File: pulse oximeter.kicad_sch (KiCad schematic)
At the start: 24 parts, among them J1 USB_C_Receptacle_USB2.0_14P, J2 Conn_01x04_Socket, J3 Conn_01x02_Socket, Q1 FS8205A, SW1 SW_Push, SW2 RESET, U1 ATMEGA328P-AU, U2 AP2112K-3.3TRG1, U3 DW01A, U4 MAX30102EFD_, U5 MCP73831-2-OT, U6 CH340C, Y1 8MHz

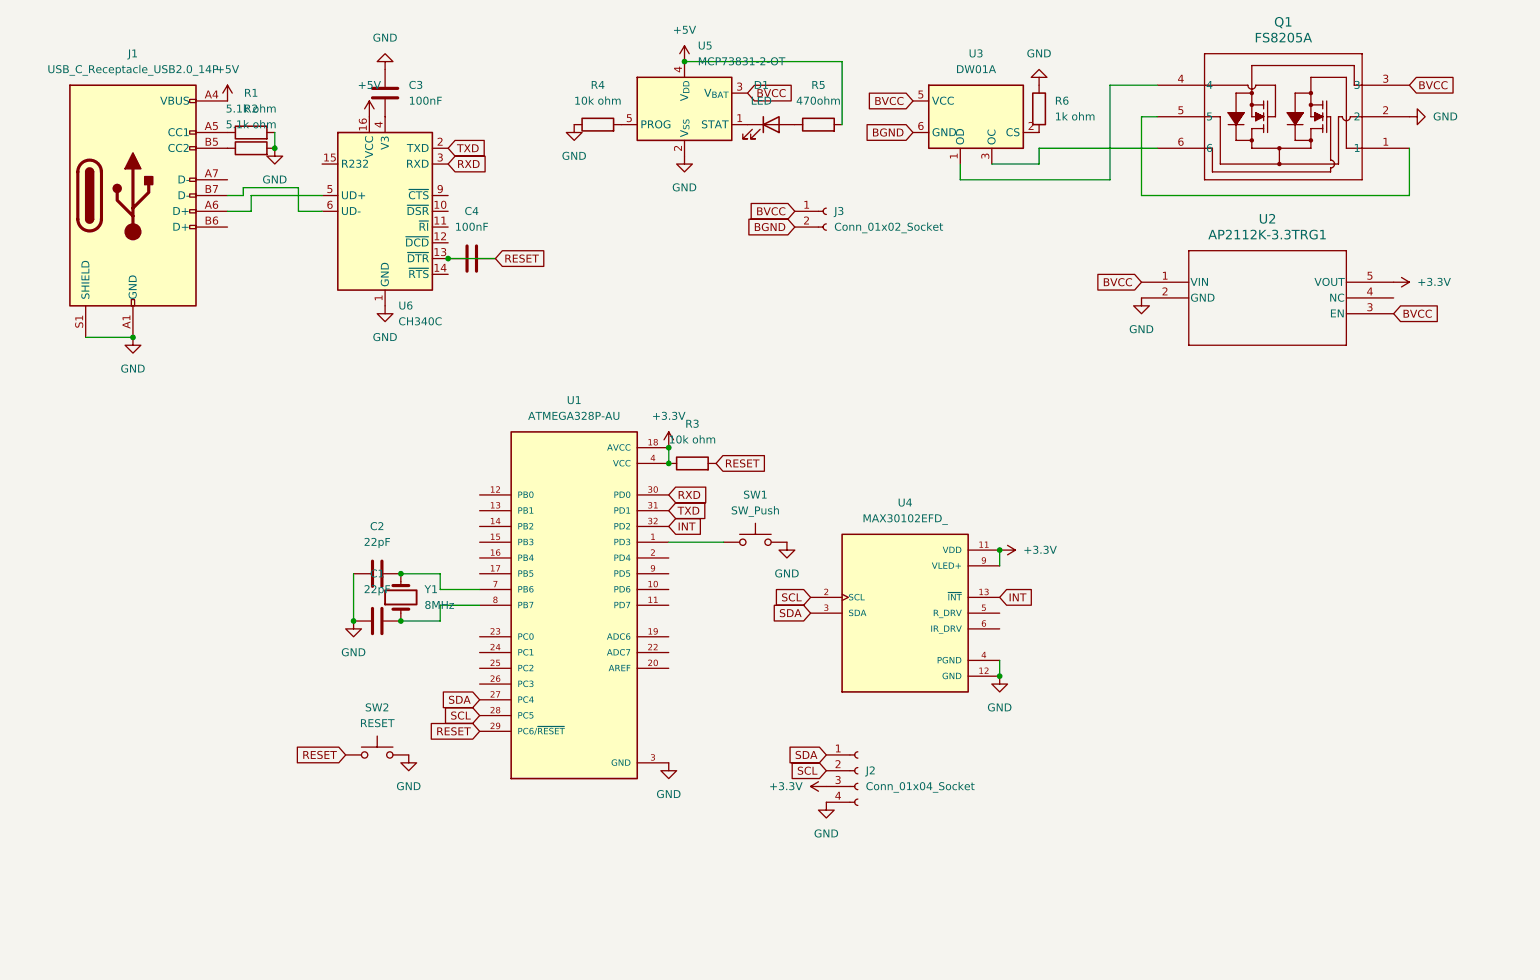
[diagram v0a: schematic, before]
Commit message: Edit PCB and Schematic
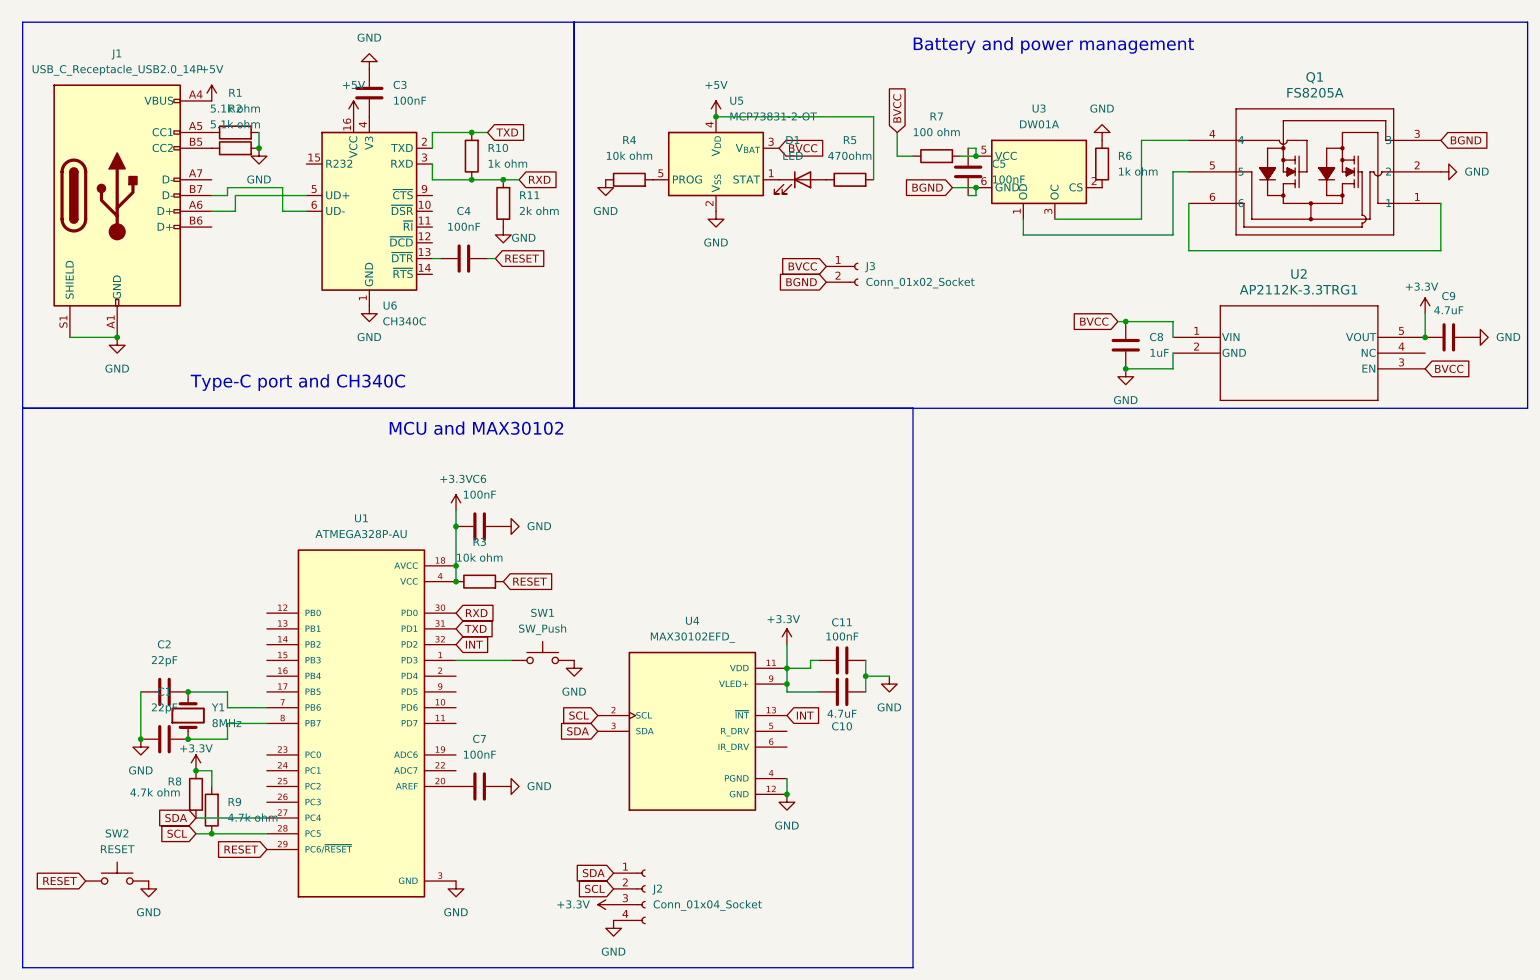
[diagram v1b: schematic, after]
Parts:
- added C10, C9: 4.7uF, Capacitor_SMD:C_0603_1608Metric, symbol Device:C
- added C11, C5, C6, C7: 100nF, Capacitor_SMD:C_0603_1608Metric, symbol Device:C
- added C8: 1uF, Capacitor_SMD:C_0603_1608Metric, symbol Device:C
- added R10: 1k ohm, Resistor_SMD:R_0603_1608Metric, symbol Device:R
- added R11: 2k ohm, Resistor_SMD:R_0603_1608Metric, symbol Device:R
- added R7: 100 ohm, Resistor_SMD:R_0603_1608Metric, symbol Device:R
- added R8, R9: 4.7k ohm, Resistor_SMD:R_0603_1608Metric, symbol Device:R
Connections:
- net +3.3V: now also C10.1, C11.1, C6.1, C9.1, R8.1, R9.2
- net BGND: now also Q1.3, C5.2
- net BVCC: now also C8.1, R7.1; no longer Q1.3, U3.5 (VCC)
- net GND: now also C10.2, C11.2, C6.2, C7.2, C8.2, C9.2, R11.1
- net RESET: no longer C4.2, U6.13 (~{DTR})
- net RXD: now also R10.1, R11.2
- net SCL: now also R9.1
- net SDA: now also R8.2
- net TXD: now also R10.2
- net at Q1.1: now also Q1.6; no longer Q1.5
- net at Q1.4: now also U3.3 (OC); no longer U3.1 (OD)
- net at U1.20 (AREF): now also C7.1
- new net: Q1.5, U3.1 (OD)
- new net: C5.1, R7.2, U3.5 (VCC)
- new net: C4.2, U6.13 (~{DTR})
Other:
- note added: "Battery and power management"
- note added: "MCU and MAX30102"
- note added: "Type-C port and CH340C"
- moved on the sheet: C1, C2, C3, C4, D1, J1, J2, J3, Q1, R1, R2, R3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
